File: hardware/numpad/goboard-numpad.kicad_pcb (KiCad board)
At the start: 2 copper layers, 77 x 105 mm, 38 parts, among them J1 Conn_02x05_Top_Bottom, J2 Conn_01x01, SW10 5, SW12 2, SW13 ., SW14 *, SW15 9, SW16 6, SW17 3, SW18 -, SW19 +, SW2 Num, SW21 Enter, SW3 7, SW4 4, SW6 1, SW7 0, SW8 /, SW9 8, U1 STM32L011F4Px

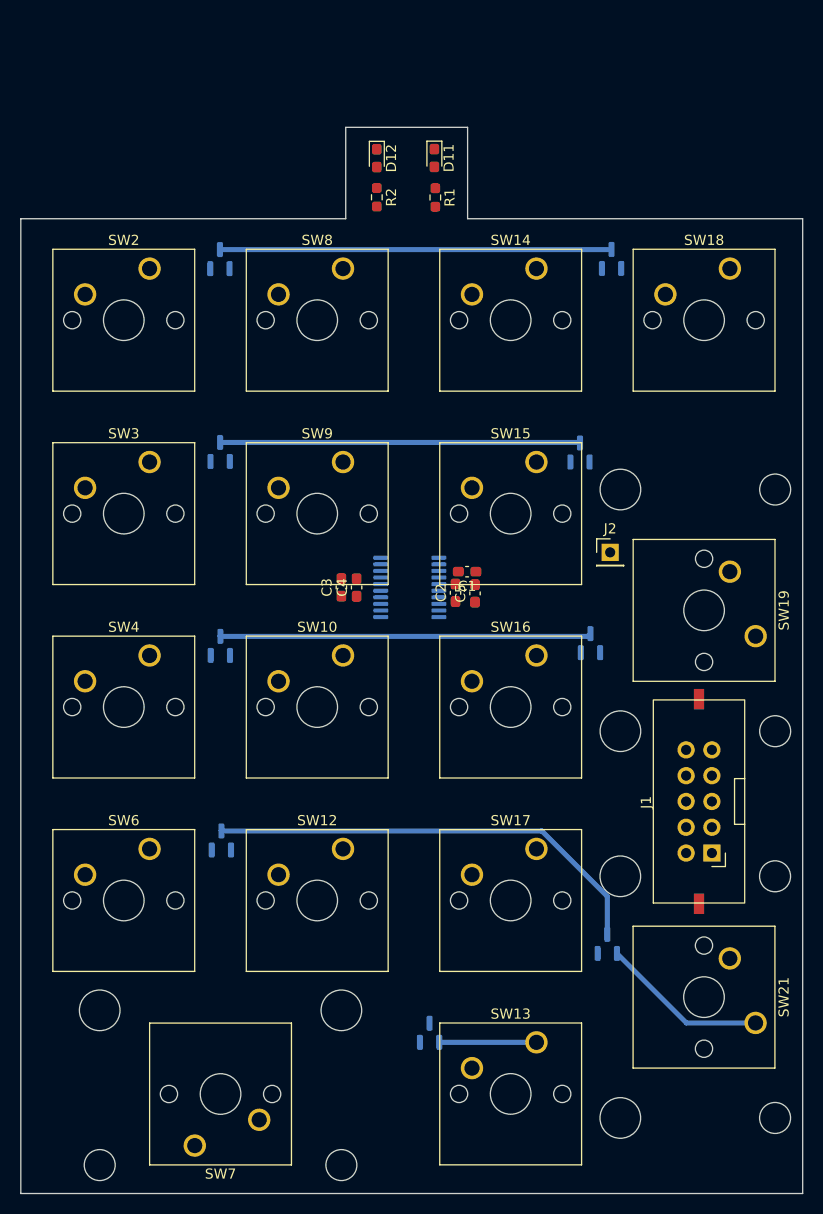
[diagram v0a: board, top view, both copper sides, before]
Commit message: Numpad: WIP: design PCB
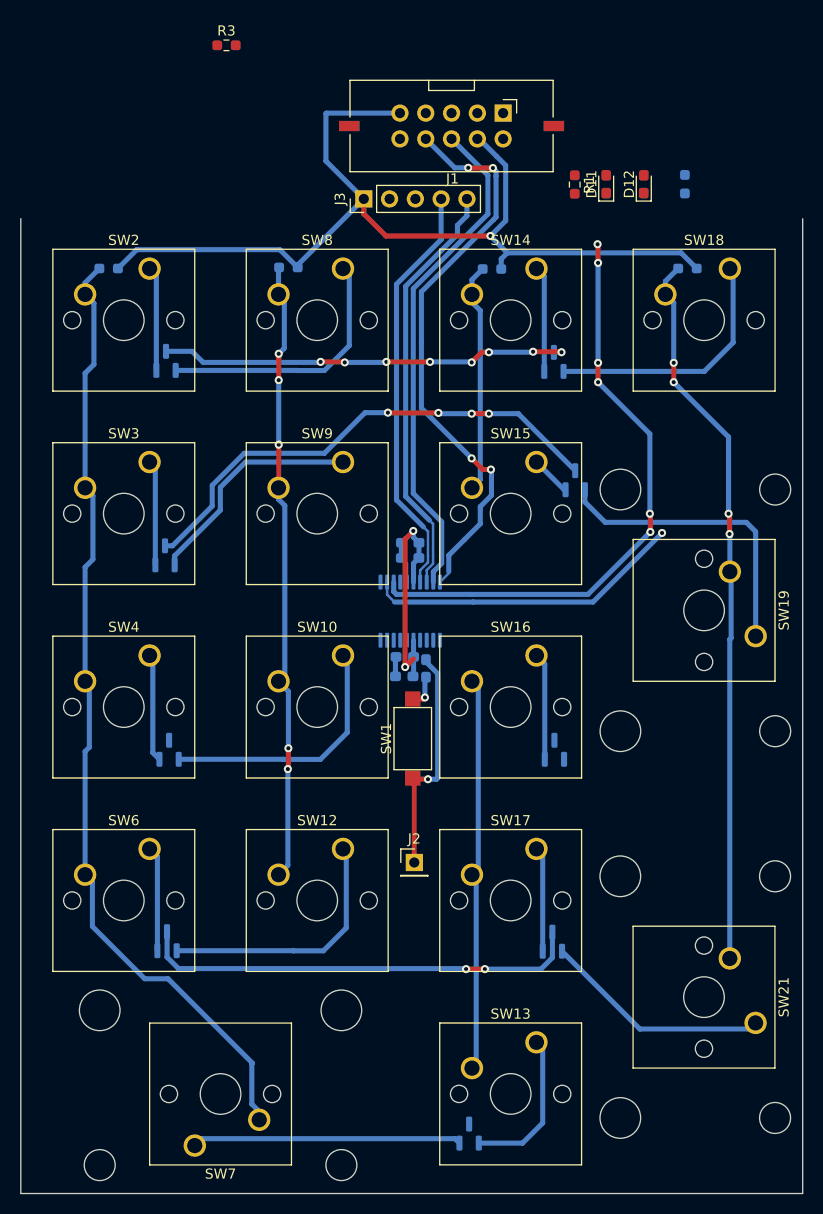
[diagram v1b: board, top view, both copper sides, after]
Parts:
- added J3: Conn_01x05, Connector_PinHeader_2.54mm:PinHeader_1x05_P2.54mm_Vertical, F.Cu at (137.8, 55.0)
- added R3: 1k, Resistor_SMD:R_0603_1608Metric_Pad0.98x0.95mm_HandSolder, F.Cu at (124.2, 39.9)
- added R4: 100k, Resistor_SMD:R_0603_1608Metric_Pad0.98x0.95mm_HandSolder, B.Cu at (112.7, 61.9)
- added R5: 100k, Resistor_SMD:R_0603_1608Metric_Pad0.98x0.95mm_HandSolder, B.Cu at (130.3, 61.8)
- added R6: 100k, Resistor_SMD:R_0603_1608Metric_Pad0.98x0.95mm_HandSolder, B.Cu at (150.4, 62.0)
- added R7: 100k, Resistor_SMD:R_0603_1608Metric_Pad0.98x0.95mm_HandSolder, B.Cu at (169.7, 61.9)
- added SW1: SW_Push, Button_Switch_SMD:SW_SPST_CK_RS282G05A3, F.Cu at (142.6, 108.2)
- C1, C2, C3, C4, C5, R2: moved to B.Cu
- SW13: value . -> dot
- SW14: value * -> times
- SW18: value - -> minus
- SW19: value + -> plus
- SW8: value / -> divide
- moved J1 75.7 mm to (151.5, 46.6), turned to 180 degrees
- moved J2 36.1 mm to (142.8, 120.4)
- moved R2 30.4 mm to (169.4, 53.6)
- moved D12 26.4 mm to (165.3, 53.6), turned to 90 degrees
- moved D11 17.1 mm to (161.7, 53.6), turned to 90 degrees
- moved R1 13.8 mm to (158.6, 53.6)
- moved D7 11.6 mm to (156.5, 71.1)
- moved D2 11.5 mm to (118.2, 90.2)
- moved D3 11.4 mm to (118.6, 109.3)
- moved D1 11.3 mm to (118.3, 71.0)
- moved D5 11.3 mm to (118.4, 128.2)
- moved D9 11.1 mm to (156.6, 109.3)
- moved C5 10.7 mm to (141.8, 102.1), turned to 0 degrees
- moved D6 10.7 mm to (148.2, 147.1)
- moved C1 10.4 mm to (143.9, 101.3), turned to -90 degrees
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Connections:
- net /mcu/COLUMN_0 renamed /Keys/COLUMN_0
- net /mcu/COLUMN_1 renamed /Keys/COLUMN_1
- net /mcu/COLUMN_2 renamed /Keys/COLUMN_2
- net /mcu/COLUMN_3 renamed /Keys/COLUMN_3
- net /mcu/COLUMN_4 renamed /Keys/COLUMN_4
- net /mcu/ROW_0 renamed /Keys/ROW_0
- net /mcu/ROW_1 renamed /Keys/ROW_1
- net /mcu/ROW_2 renamed /Keys/ROW_2
- net /mcu/ROW_3 renamed /Keys/ROW_3
- D9 pad 1: Net-(D9-Pad1) -> unconnected-(D9-Pad1)
- J1 pad 10: no_connect_40 -> unconnected-(J1-Pad10)
- J1 pad 3: no_connect_41 -> unconnected-(J1-Pad3)
- J1 pad 5: no_connect_42 -> unconnected-(J1-Pad5)
- U1 pad 11: /mcu/COLUMN_5 -> unconnected-(U1-Pad11)
- U1 pad 17: /mcu/UART_TX -> /UART_TX
- U1 pad 18: /mcu/UART_RX -> /UART_RX
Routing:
- net VCC: track 0.00 -> 120.9 mm, vias 0 -> 3
- net /Keys/ROW_0: track 0.00 -> 94.6 mm
- net /Keys/ROW_3: track 0.00 -> 71.2 mm, vias 0 -> 4
- net /Keys/ROW_2: track 0.00 -> 61.6 mm
- net /Keys/ROW_1: track 0.00 -> 61.6 mm, vias 0 -> 5
- net /mcu/LED_POWER: track 0.00 -> 59.4 mm, vias 0 -> 6
- net /SWDCLK: track 0.00 -> 57.2 mm, vias 0 -> 4
- net /SWDIO: track 0.00 -> 49.7 mm
- net /UART_RX: track 0.00 -> 41.6 mm
- net /UART_TX: track 0.00 -> 41.2 mm
- net /Keys/COLUMN_2: track 36.6 -> 0.00 mm
- net /mcu/LED_NUMLOCK: track 0.00 -> 31.4 mm, vias 0 -> 1
- net Net-(D8-Pad1): track 0.00 -> 29.5 mm
- net Net-(D6-Pad2): track 0.01 -> 26.5 mm
- net Net-(D1-Pad1): track 0.00 -> 26.0 mm
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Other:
- board size 77 x 105 mm -> 77 x 96 mm
